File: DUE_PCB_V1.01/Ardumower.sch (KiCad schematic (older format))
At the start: 54 parts, among them J1 I2C_1, J10 Bumper Left, J11 Bumper Right, J12 P_Left, J13 P_Right, J14 Sonar_R, J15 Sonar_C, J16 Sonar_L, J17 US1, J18 US2, J19 US3, J2 I2C_2, J20 Button, J21 5V IN, J22 Remote, J23 PCB_2, J24 3.3V IN, J25 Ser0, J26 Ser1, J27 Ser2 (ESP32), J28 GPS_TX/GPS_RX, J3 I2C_3, J4 DS3231 RTC, J5 9V IN, J6 Drop_Left, J7 Drop_Right, J8 Tilt, J9 Rain

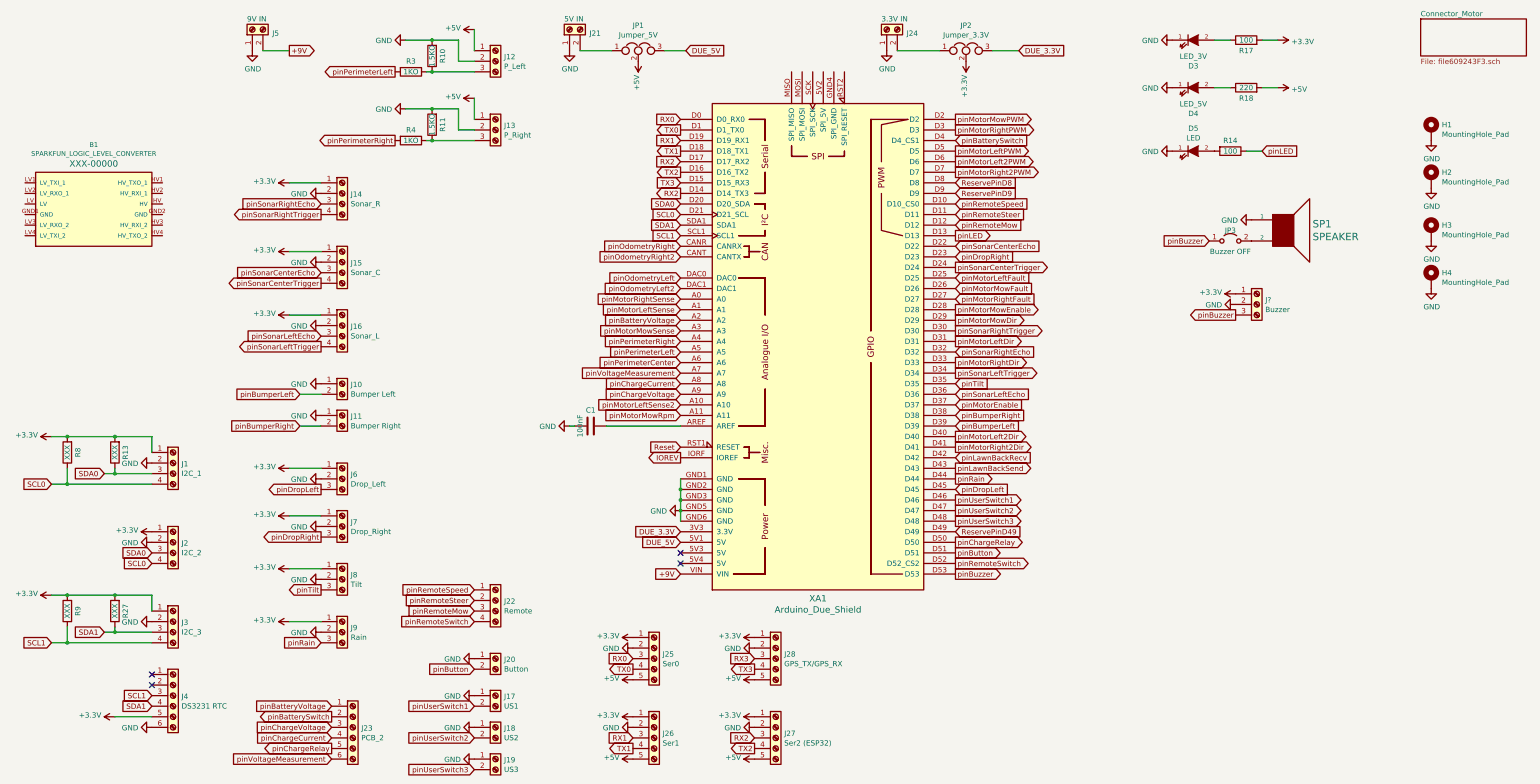
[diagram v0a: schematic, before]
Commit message: Change I2C Names
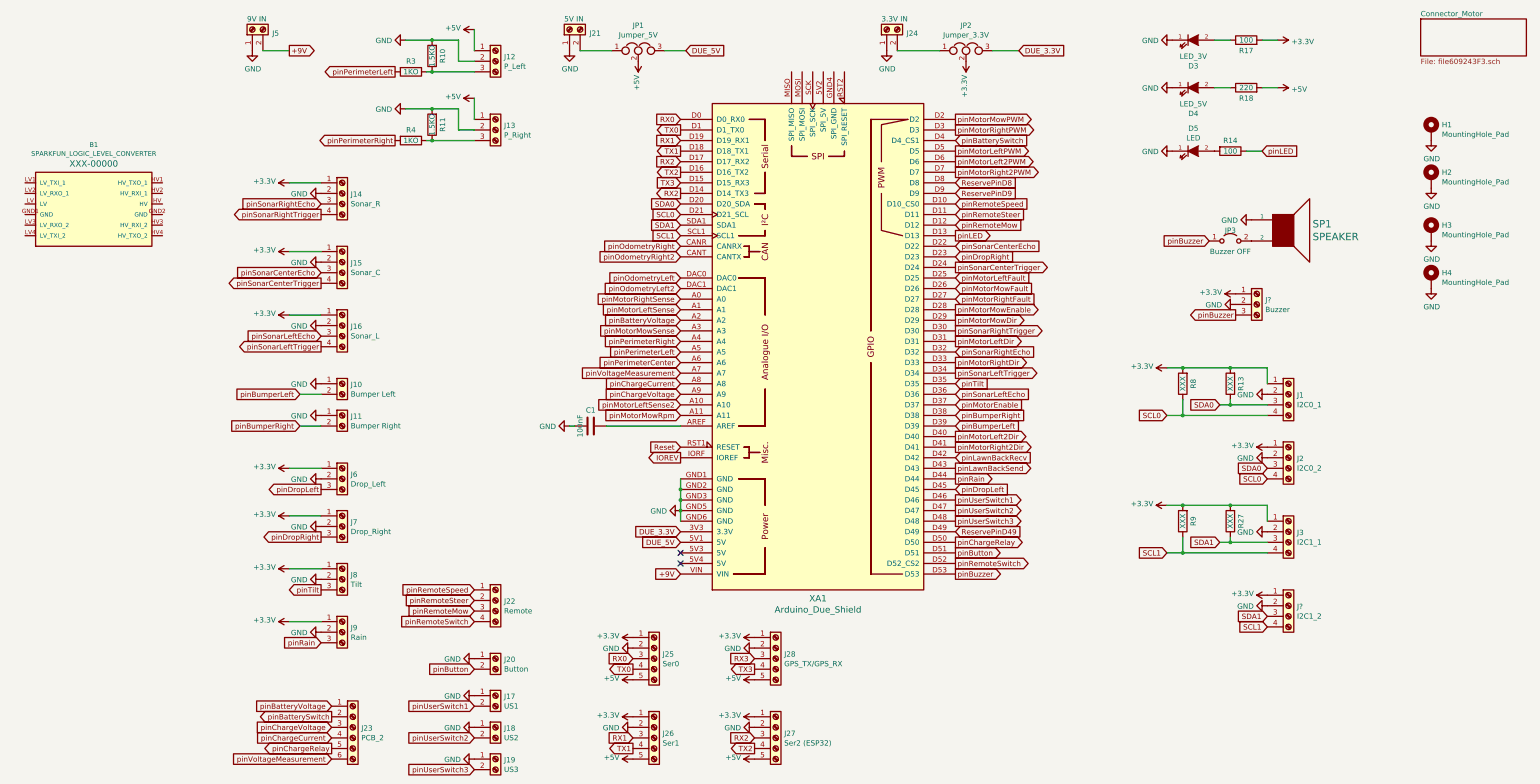
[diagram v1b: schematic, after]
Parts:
- removed J4: DS3231 RTC, Connector_PinHeader_2.54mm:PinHeader_1x06_P2.54mm_Vertical, symbol Connector:Screw_Terminal_01x06
- added J?: I2C1_2, Connector_PinHeader_2.54mm:PinHeader_1x04_P2.54mm_Vertical, symbol Connector:Screw_Terminal_01x04
- J1: value I2C_1 -> I2C0_1
- J2: value I2C_2 -> I2C0_2
- J3: value I2C_3 -> I2C1_1
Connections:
- net +3V3: now also J?.1 (Pin_1)
- net GND: now also J?.2 (Pin_2)
- net SCL1: now also J?.4 (Pin_4)
- net SDA1: now also J?.3 (Pin_3)
- no-connect marks 4 -> 2
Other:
- moved on the sheet: J1, J2, J3, R13, R27, R8, R9
